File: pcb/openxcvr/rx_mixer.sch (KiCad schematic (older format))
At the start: 16 parts, among them T1 BN43-24023, U4 LM4562, U5 FST5253

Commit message: update rev0.2 PCB
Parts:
- added C51: 100n, Capacitor_SMD:C_0805_2012Metric, symbol Device:C
- added J8: Conn_01x03_Male, Connector_PinHeader_2.54mm:PinHeader_1x03_P2.54mm_Vertical, symbol Connector:Conn_01x03_Male
- T1: value BN43-24023 -> BN43-2402; symbol xcvr_components:cx2074NL -> RADIO-rescue:cx2074NL-xcvr_components
- U5: symbol xcvr_components:FST5253 -> RADIO-rescue:FST5253-xcvr_components
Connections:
- wire segments 71 -> 81
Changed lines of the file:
@@
 Connection ~ 8750 4800
 Connection ~ 8750 5200
+Connection ~ 9450 3600
+Connection ~ 9450 5200
 Wire Wire Line
 	1050 4200 1400 4200
@@
 	3600 5100 3600 5350
 Wire Wire Line
+	4000 1150 4000 1300
+Wire Wire Line
+	4000 1600 4000 1700
+Wire Wire Line
 	4000 4100 4300 4100
 Wire Wire Line
@@
 	8750 5200 9000 5200
 Wire Wire Line
-	9300 3600 9600 3600
-Wire Wire Line
-	9300 5200 9600 5200
+	9100 4200 9450 4200
+Wire Wire Line
+	9100 4300 9800 4300
+Wire Wire Line
+	9100 4400 9450 4400
+Wire Wire Line
+	9300 3600 9450 3600
+Wire Wire Line
+	9300 5200 9450 5200
+Wire Wire Line
+	9450 3600 9600 3600
+Wire Wire Line
+	9450 4200 9450 3600
+Wire Wire Line
+	9450 4400 9450 5200
+Wire Wire Line
+	9450 5200 9600 5200
+Wire Wire Line
+	9800 4300 9800 4600
 Text Notes 2200 3450 2    50   ~ 0
 Primary 4T Unifilar\nSecondary 2T Bifilar\n
@@
 $EndComp
 $Comp
+L power:+5V #PWR0102
+U 1 1 5ECD0B83
+P 4000 1150
+F 0 "#PWR0102" H 4000 1000 50  0001 C CNN
+F 1 "+5V" H 4015 1323 50  0000 C CNN
+F 2 "" H 4000 1150 50  0001 C CNN
+F 3 "" H 4000 1150 50  0001 C CNN
+	1    4000 1150
+	1    0    0    -1
+$EndComp
+$Comp
 L power:+2V5 #PWR050
 U 1 1 5E6C5245
@@
 $EndComp
 $Comp
+L power:GND #PWR0103
+U 1 1 5ECD0B93
+P 4000 1700
+F 0 "#PWR0103" H 4000 1450 50  0001 C CNN
+F 1 "GND" H 4005 1527 50  0000 C CNN
+F 2 "" H 4000 1700 50  0001 C CNN
+F 3 "" H 4000 1700 50  0001 C CNN
+	1    4000 1700
+	1    0    0    -1
+$EndComp
+$Comp
 L power:GND #PWR048
 U 1 1 5E73DEF2
@@
 F 3 "" H 6150 5750 50  0001 C CNN
 	1    6150 5750
+	1    0    0    -1
+$EndComp
+$Comp
+L power:GND #PWR0105
+U 1 1 5EDC0D6C
+P 9800 4600
+F 0 "#PWR0105" H 9800 4350 50  0001 C CNN
+F 1 "GND" H 9805 4427 50  0000 C CNN
+F 2 "" H 9800 4600 50  0001 C CNN
+F 3 "" H 9800 4600 50  0001 C CNN
+	1    9800 4600
 	1    0    0    -1
 $EndComp
@@
 $EndComp
 $Comp
+L Device:C C51
+U 1 1 5ECD0BA5
+P 4000 1450
+F 0 "C51" H 4115 1495 50  0000 L CNN
+F 1 "100n" H 4115 1405 50  0000 L CNN
+F 2 "Capacitor_SMD:C_0805_2012Metric" H 4038 1300 50  0001 C CNN
+F 3 "~" H 4000 1450 50  0001 C CNN
+	1    4000 1450
+	1    0    0    -1
+$EndComp
+$Comp
 L Device:C C21
 U 1 1 5E72F21F
@@
 $EndComp
 $Comp
+L Connector:Conn_01x03_Male J8
+U 1 1 5EDBE7DA
+P 8900 4300
+F 0 "J8" H 9008 4579 50  0000 C CNN
+F 1 "Conn_01x03_Male" H 9008 4488 50  0000 C CNN
+F 2 "Connector_PinHeader_2.54mm:PinHeader_1x03_P2.54mm_Vertical" H 8900 4300 50  0001 C CNN
+F 3 "~" H 8900 4300 50  0001 C CNN
+	1    8900 4300
+	1    0    0    -1
+$EndComp
+$Comp
 L Amplifier_Operational:LM4562 U4
 U 2 1 5E26166E
@@
 $EndComp
 $Comp
-L xcvr_components:cx2074NL T1
+L RADIO-rescue:cx2074NL-xcvr_components T1
 U 1 1 5E6894D6
 P 1800 4000
 F 0 "T1" H 1800 4379 50  0000 C CNN
-F 1 "BN43-24023" H 1800 4288 50  0000 C CNN
+F 1 "BN43-2402" H 1800 4288 50  0000 C CNN
 F 2 "openxcvr:bn43-2402-transformer" H 1800 4000 50  0001 C CNN
 F 3 "https://datasheet.octopart.com/CX2074NL-Pulse-datasheet-123678.pdf" H 1800 4000 50  0001 C CNN
@@
 $EndComp
 $Comp
-L xcvr_components:FST5253 U5
+L RADIO-rescue:FST5253-xcvr_components U5
 U 1 1 5E2AF6E6
 P 3600 4500
+AR Path="/5E2AF6E6" Ref="U5"  Part="1"
+AR Path="/5E35BCF5/5E2AF6E6" Ref="U5"  Part="1"
 F 0 "U5" H 4000 5200 50  0000 C CNN
 F 1 "FST5253" H 4000 5100 50  0000 C CNN

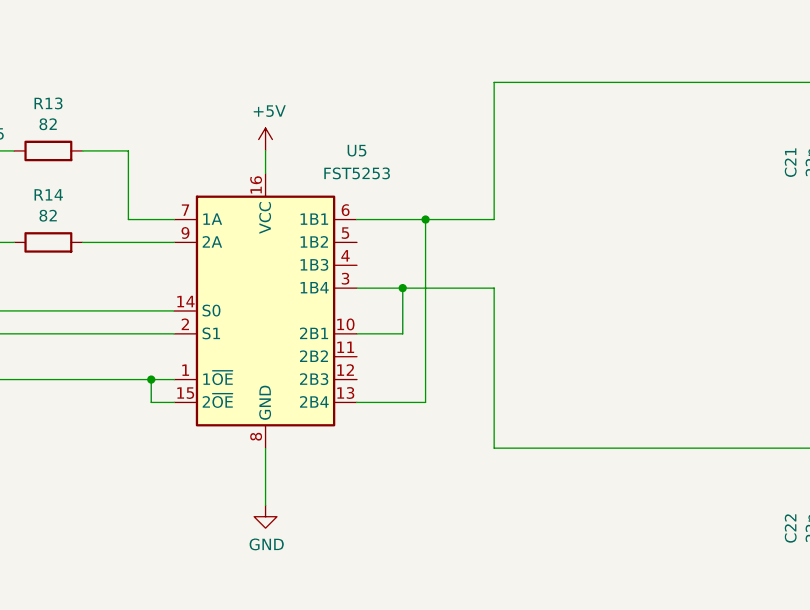
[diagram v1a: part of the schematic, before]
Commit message: Review and update schematic
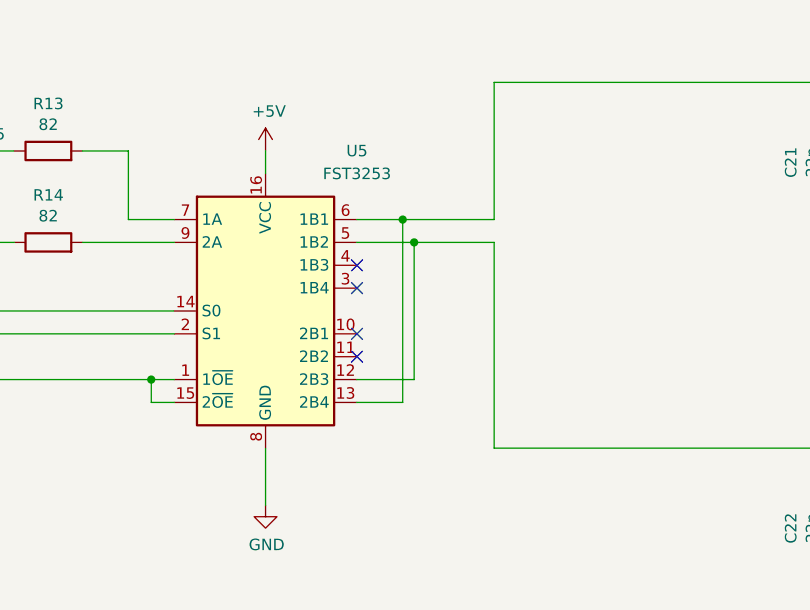
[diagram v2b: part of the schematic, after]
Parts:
- U5: value FST5253 -> FST3253
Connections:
- no-connect marks 0 -> 4
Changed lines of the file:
@@
 $EndDescr
 Connection ~ 3100 4800
-Connection ~ 4200 4400
-Connection ~ 4300 4100
+Connection ~ 4200 4100
+Connection ~ 4250 4200
 Connection ~ 6150 3500
 Connection ~ 6150 5100
@@
 Connection ~ 9450 3600
 Connection ~ 9450 5200
+NoConn ~ 4000 4300
+NoConn ~ 4000 4400
+NoConn ~ 4000 4600
+NoConn ~ 4000 4700
 Wire Wire Line
 	1050 4200 1400 4200
@@
 	4000 1600 4000 1700
 Wire Wire Line
-	4000 4100 4300 4100
-Wire Wire Line
-	4000 4400 4200 4400
-Wire Wire Line
-	4000 4600 4200 4600
-Wire Wire Line
-	4000 4900 4300 4900
-Wire Wire Line
-	4200 4400 4600 4400
-Wire Wire Line
-	4200 4600 4200 4400
-Wire Wire Line
-	4300 4100 4300 4900
-Wire Wire Line
-	4300 4100 4600 4100
+	4000 4100 4200 4100
+Wire Wire Line
+	4000 4200 4250 4200
+Wire Wire Line
+	4000 4800 4250 4800
+Wire Wire Line
+	4000 4900 4200 4900
+Wire Wire Line
+	4200 4100 4600 4100
+Wire Wire Line
+	4200 4900 4200 4100
+Wire Wire Line
+	4250 4200 4600 4200
+Wire Wire Line
+	4250 4800 4250 4200
 Wire Wire Line
 	4600 3500 6150 3500
@@
 	4600 4100 4600 3500
 Wire Wire Line
-	4600 4400 4600 5100
+	4600 4200 4600 5100
 Wire Wire Line
 	4600 5100 6150 5100
@@
 AR Path="/5E35BCF5/5E2AF6E6" Ref="U5"  Part="1"
 F 0 "U5" H 4000 5200 50  0000 C CNN
-F 1 "FST5253" H 4000 5100 50  0000 C CNN
+F 1 "FST3253" H 4000 5100 50  0000 C CNN
 F 2 "Package_SO:SOIC-16_3.9x9.9mm_P1.27mm" H 3600 4500 50  0001 C CNN
 F 3 "http://www.ti.com/lit/gpn/sn74cbt3253" H 3600 4500 50  0001 C CNN
